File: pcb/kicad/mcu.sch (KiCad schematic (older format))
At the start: 25 parts, among them J2 SD_CARD, J3 USB_MINIB, P1 CONN_7X2, P2 CONN_2, U11 LPC1754, X1 12MHz, X2 32.768kHz

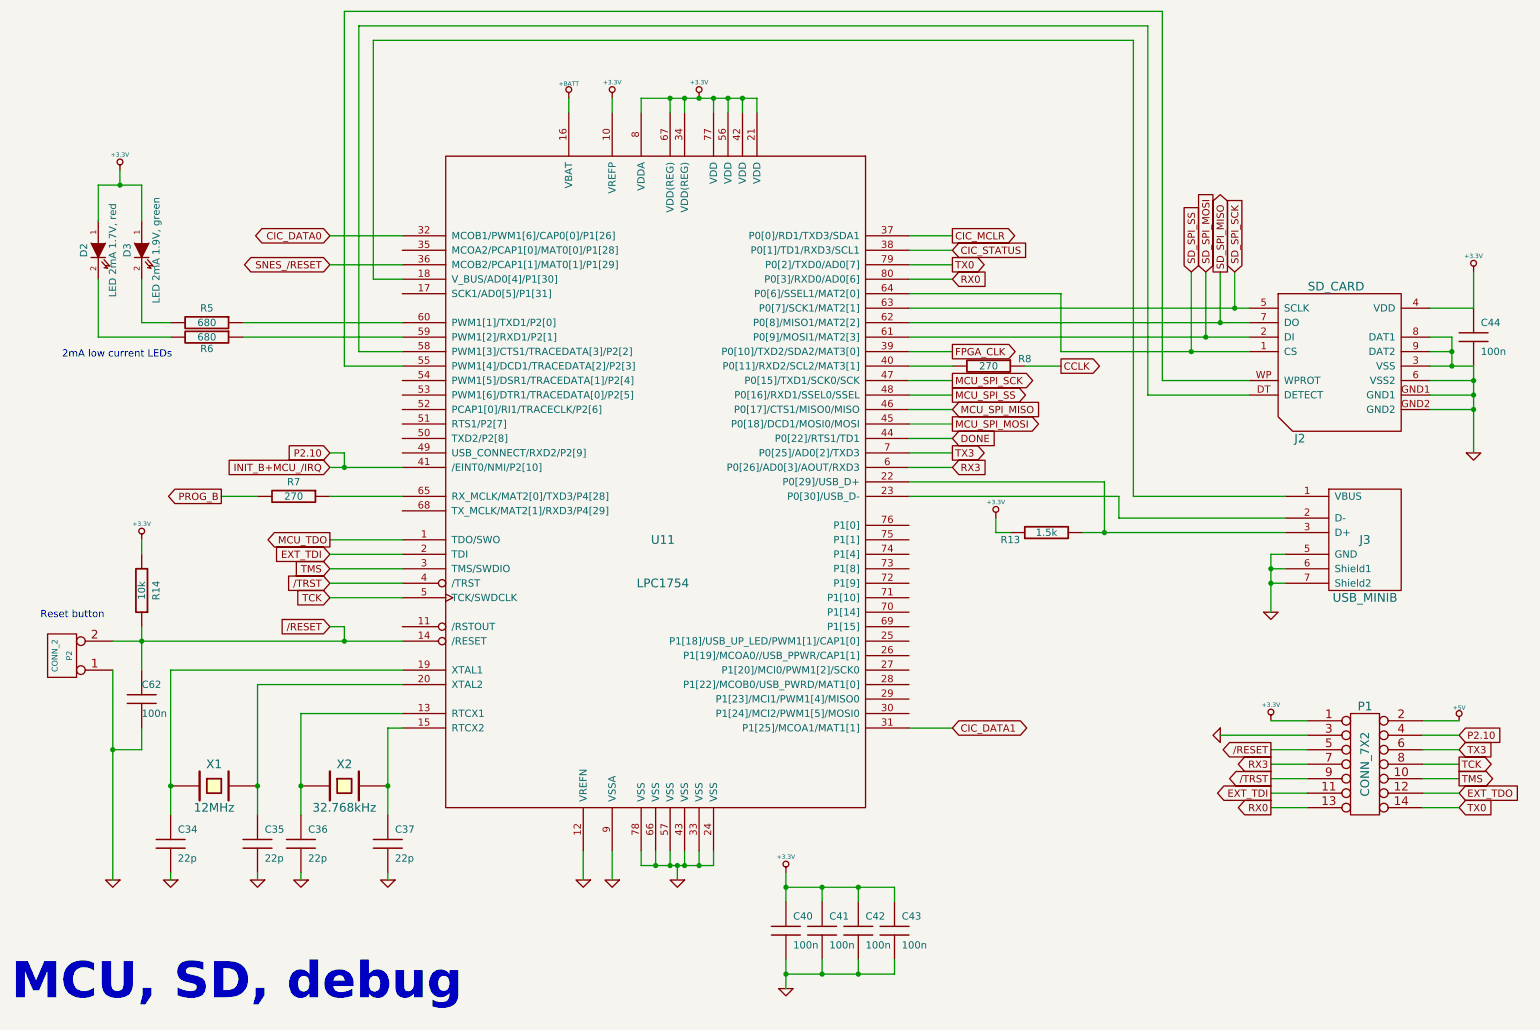
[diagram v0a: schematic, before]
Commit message: pcb wip
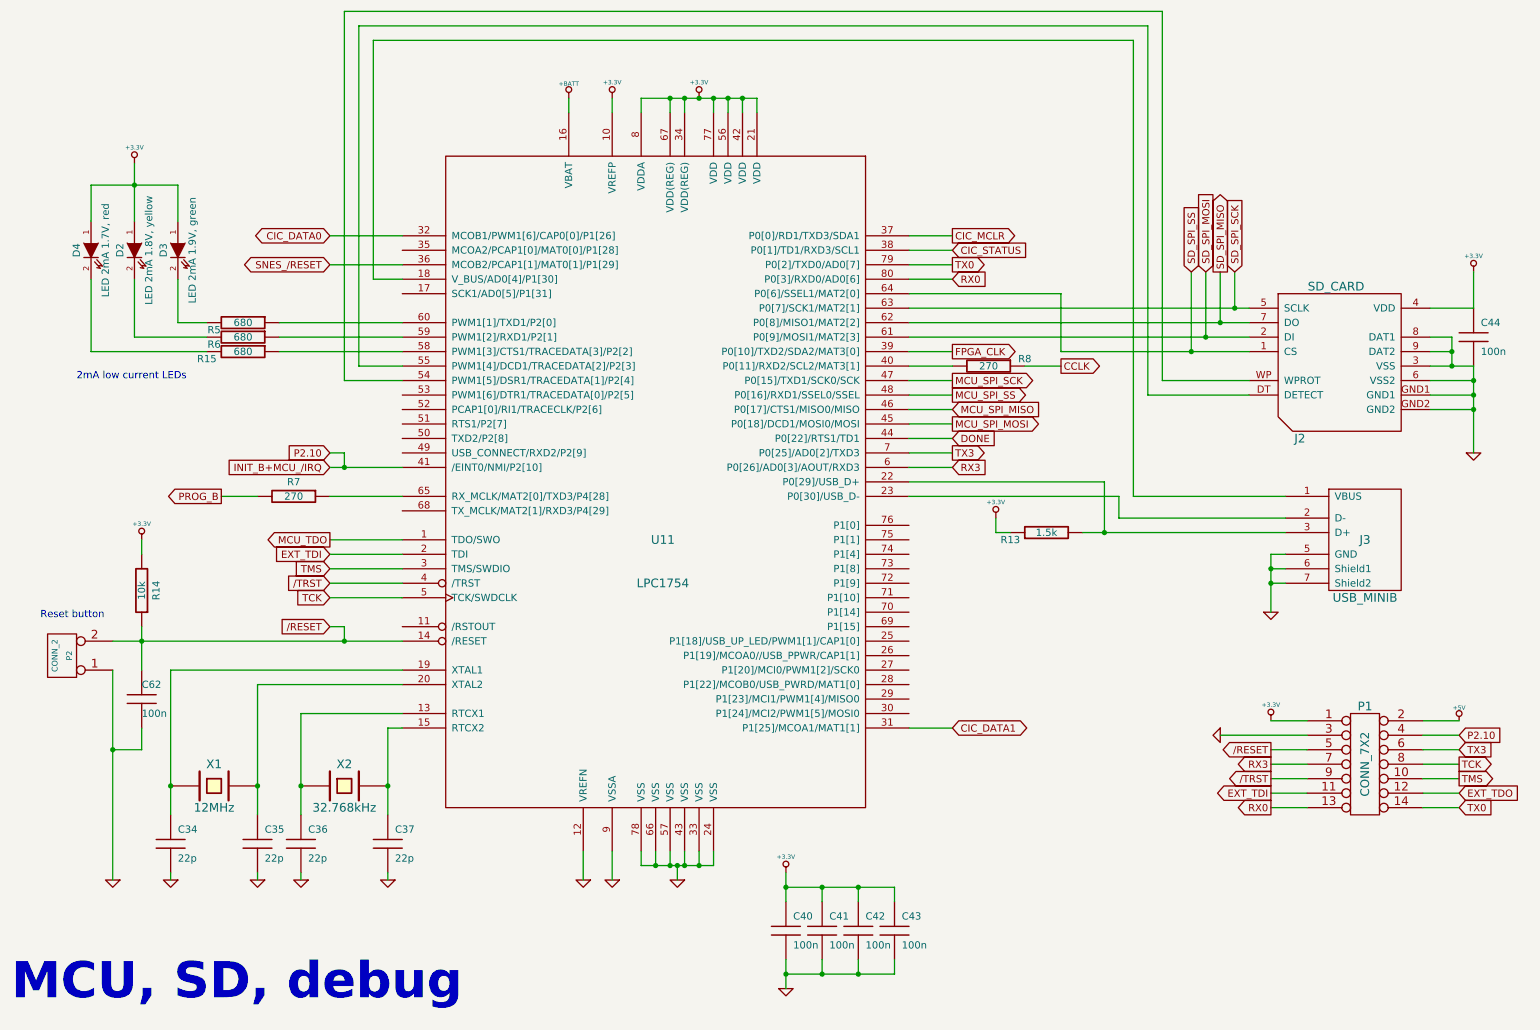
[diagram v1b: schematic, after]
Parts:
- added D4: LED 2mA 1.7V, red, symbol LED
- added R15: 680, symbol R
- D2: value LED 2mA 1.7V, red -> LED 2mA 1.8V, yellow
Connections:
- net +3.3V: now also D4.1 (A)
- net at U11.54 (PWM1[5]/DSR1/TRACEDATA[1]/P2[4]): now also J2.WP (WPROT)
- net at U11.55 (PWM1[4]/DCD1/TRACEDATA[2]/P2[3]): now also J2.DT (DETECT); no longer J2.WP (WPROT)
- net at U11.58 (PWM1[3]/CTS1/TRACEDATA[3]/P2[2]): now also R15.1; no longer J2.DT (DETECT)
- new net: D4.2 (K), R15.2
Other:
- moved on the sheet: D2, D3, R5, R6
